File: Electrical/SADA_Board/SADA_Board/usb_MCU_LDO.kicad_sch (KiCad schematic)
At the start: 23 parts, among them IC1 TPS25940LRVCR, J14 USB_B_Micro, Q1 NVR5198NLT1G, Q2 NVR5198NLT1G, U6 NCV68261MTWAITBG, U8 NCV68261MTWAITBG

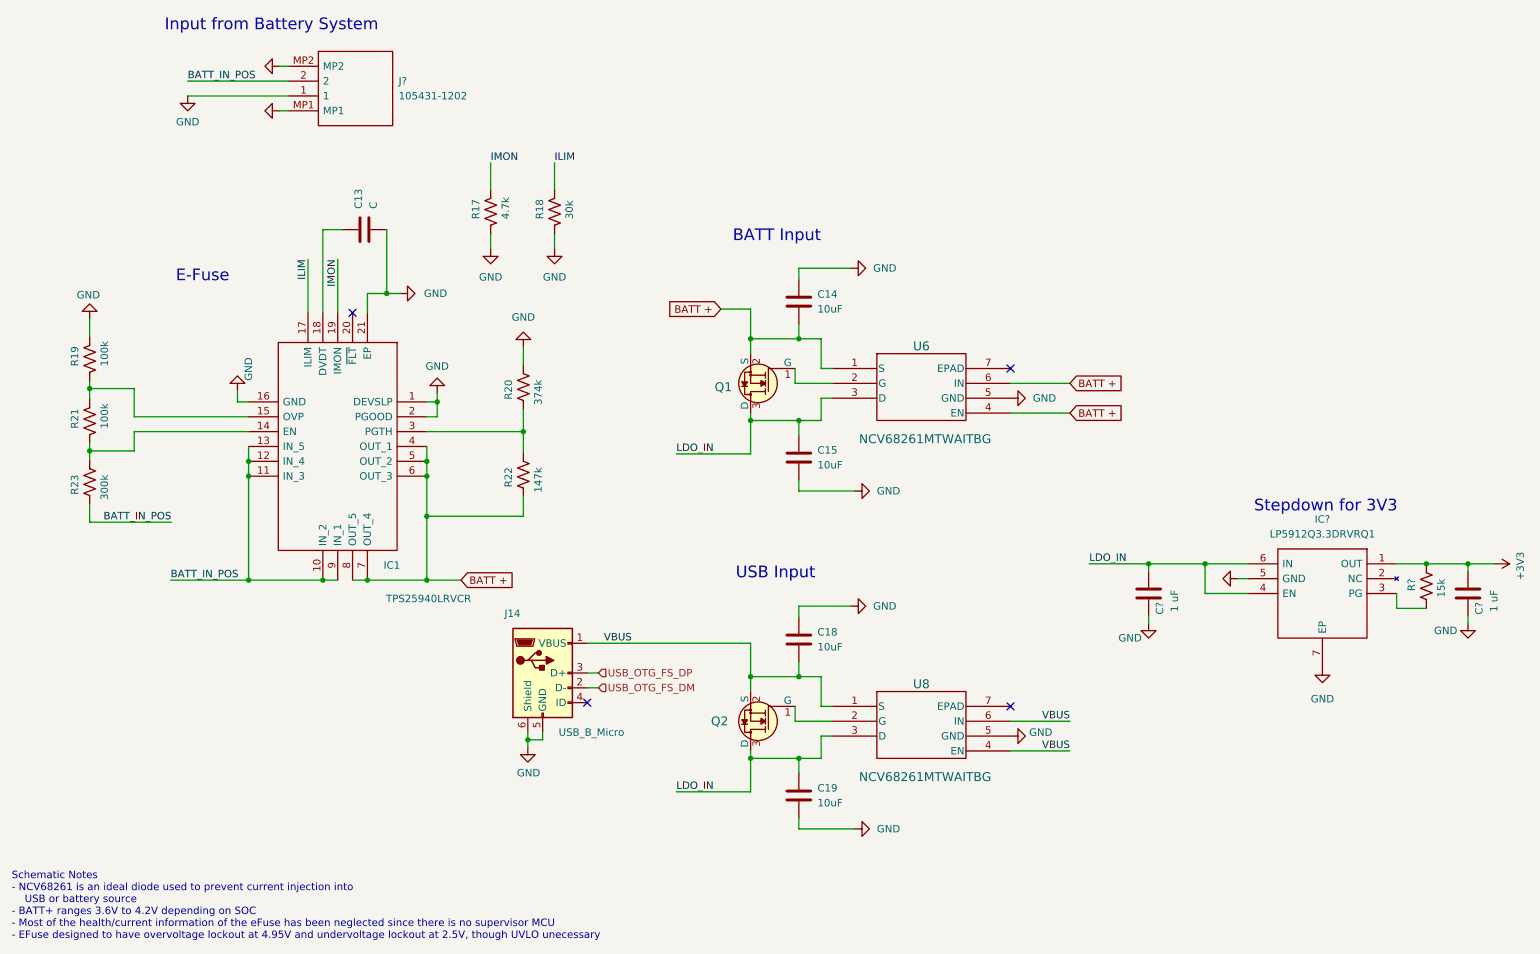
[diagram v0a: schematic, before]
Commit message: Pre-Design Review II
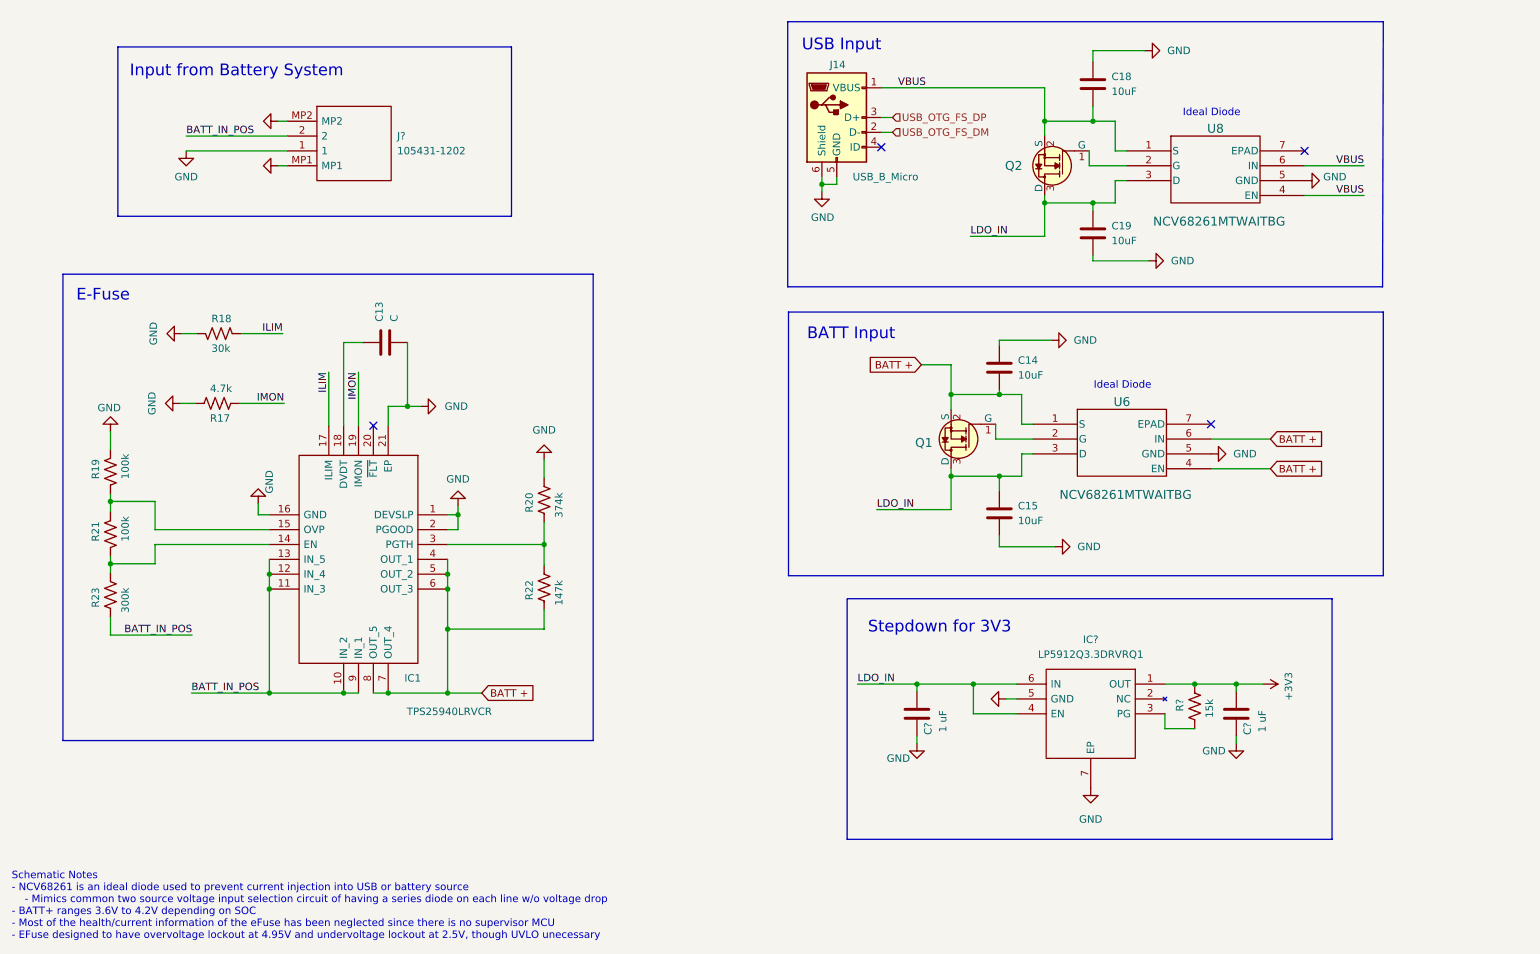
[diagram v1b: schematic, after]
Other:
- note added: "Ideal Diode"
- note added: "Schematic Notes - NCV68261 is an ideal diode used to prevent current injection into USB or battery source - Mimics common two source voltage input selection circuit of having a series diode on each line w/o voltage drop - BATT+ ranges 3.6V to 4.2V depending on SOC - Most of the health/current information of the eFuse has been neglected since there is no supervisor MCU - EFuse designed to have ove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"
- note removed: "Schematic Notes - NCV68261 is an ideal diode used to prevent current injection into USB or battery source - BATT+ ranges 3.6V to 4.2V depending on SOC - Most of the health/current information of the eFuse has been neglected since there is no supervisor MCU - EFuse designed to have overvoltage lockout at 4.95V and undervoltage lockout at 2.5V, though UVLO unecessary"
- moved on the sheet: C13, C14, C15, C18, C19, C?, IC1, IC?, J14, J?, Q1, Q2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

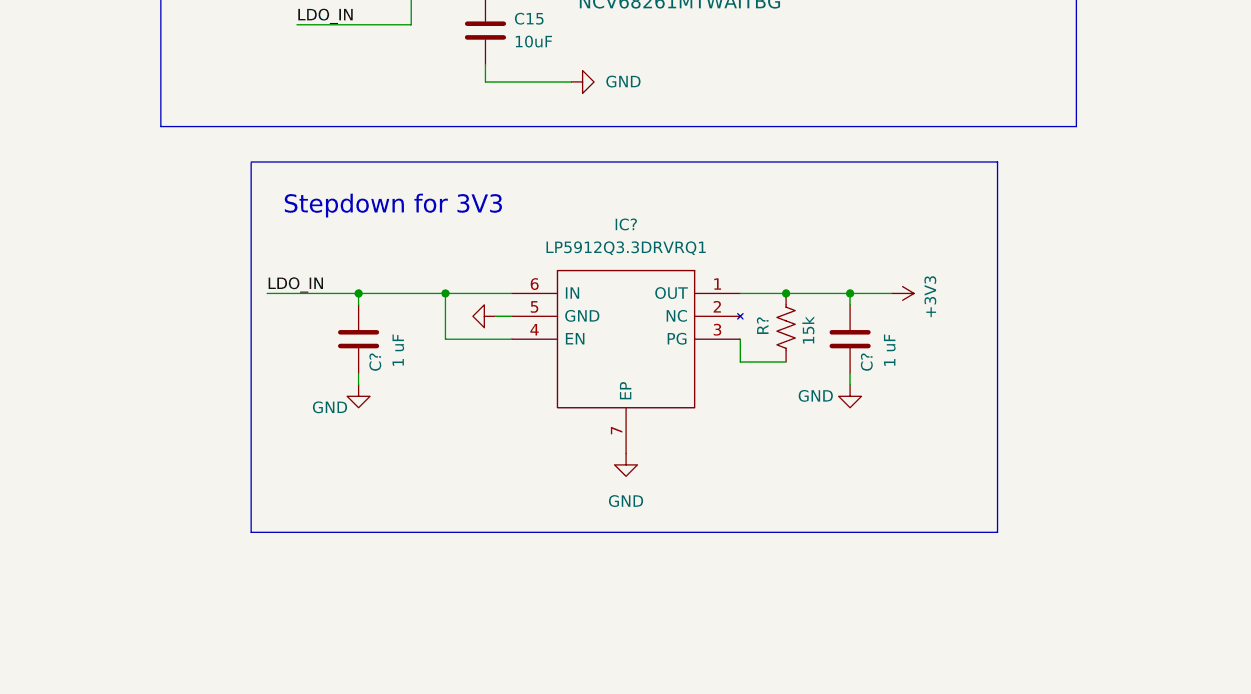
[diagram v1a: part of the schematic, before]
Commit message: Pre-passive retainment change
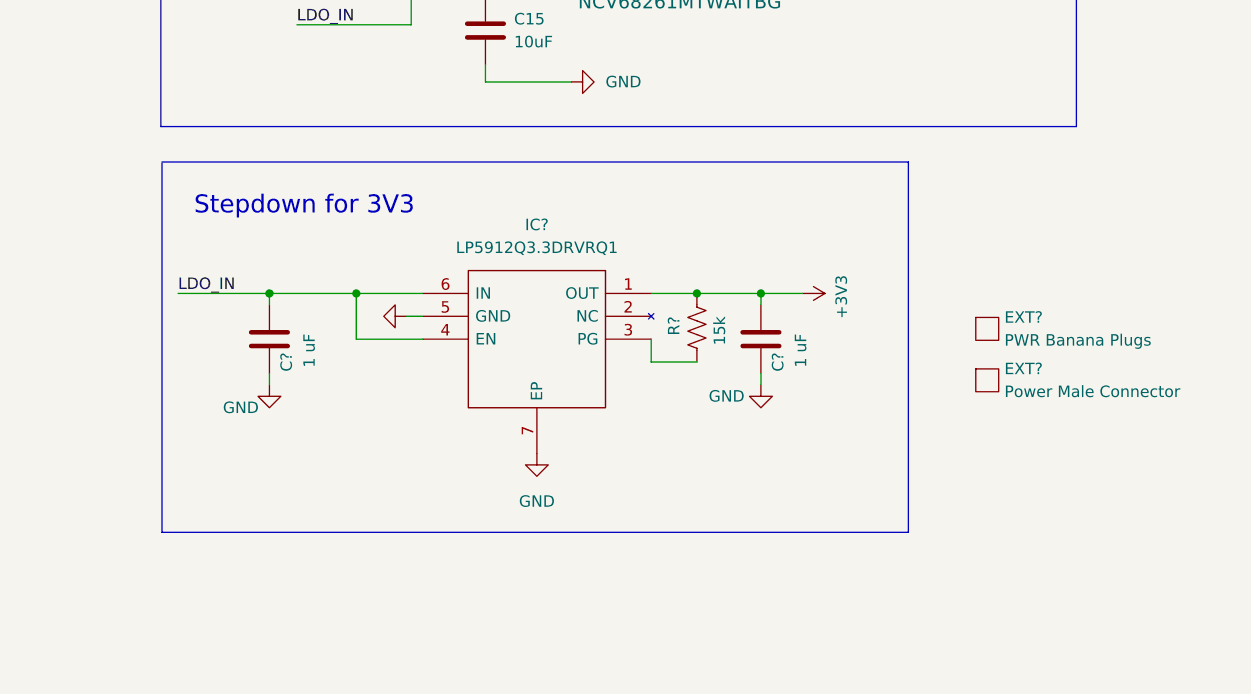
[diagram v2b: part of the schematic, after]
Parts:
- added EXT?: PWR Banana Plugs, 0_custom:EXT_no_footprint, symbol 0_custom:{lt}name{gt}
- added EXT?: Power Male Connector, 0_custom:EXT_no_footprint, symbol 0_custom:{lt}name{gt}
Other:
- moved on the sheet: C?, IC?, R?
